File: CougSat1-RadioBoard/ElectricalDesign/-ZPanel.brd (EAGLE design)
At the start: 96 x 96 mm, 46 parts, among them J1 High Gain Antenna, J2 Deployables, J3 High Gain +, J4 ADCS, J5 Flap +X, J6 Flap -X, J7 Flap +Y, J8 Flap -Y, U1 AD7291, U3 AD8515

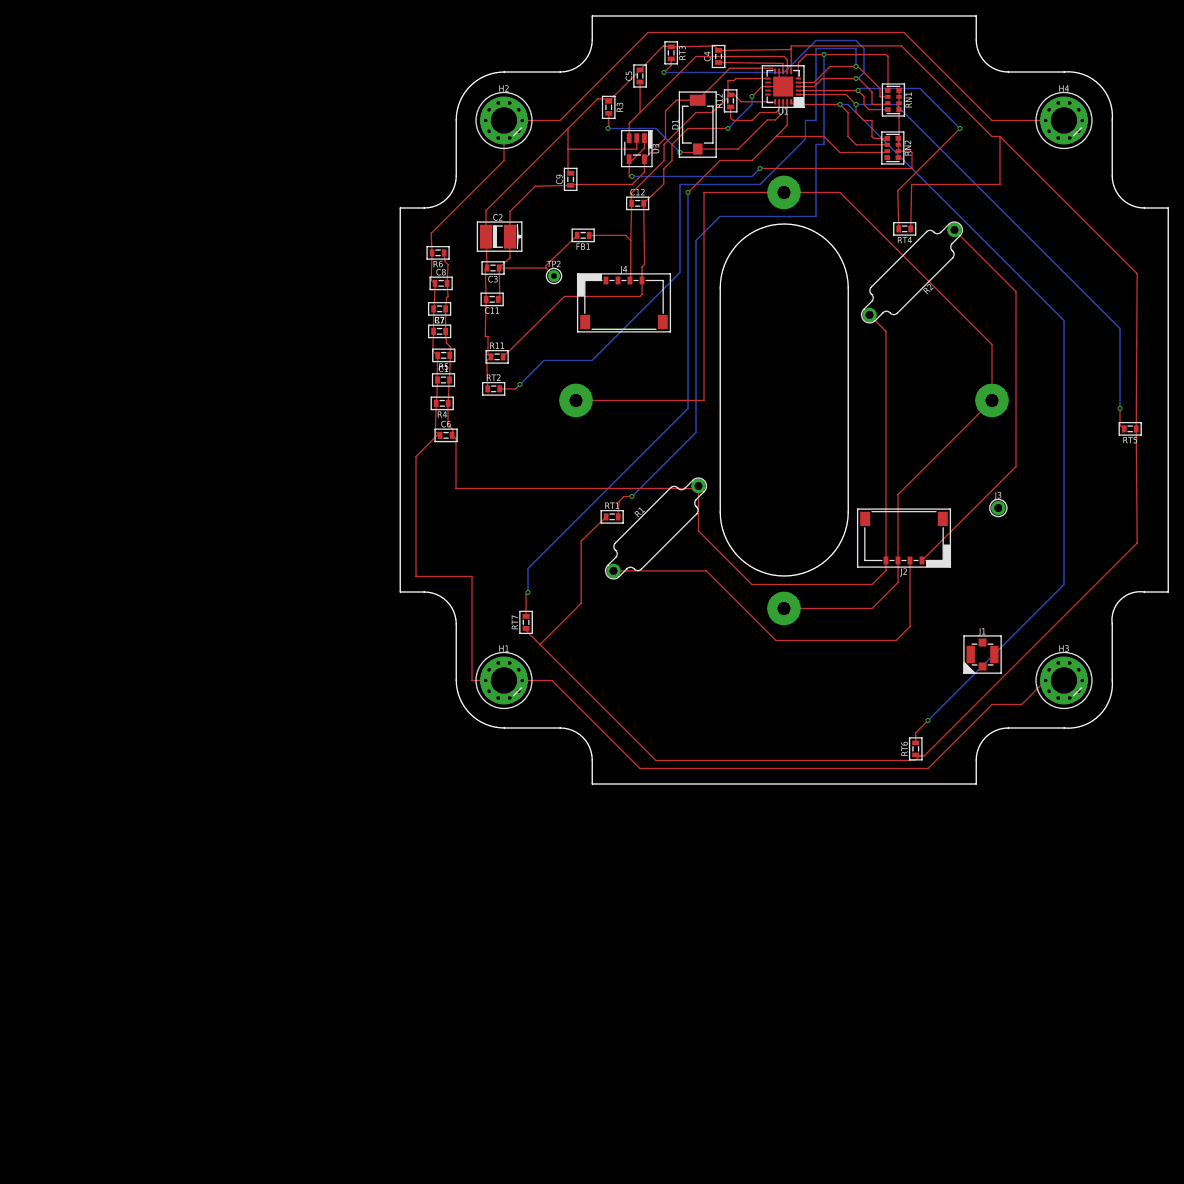
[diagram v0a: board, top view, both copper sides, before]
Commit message: Laid out RF
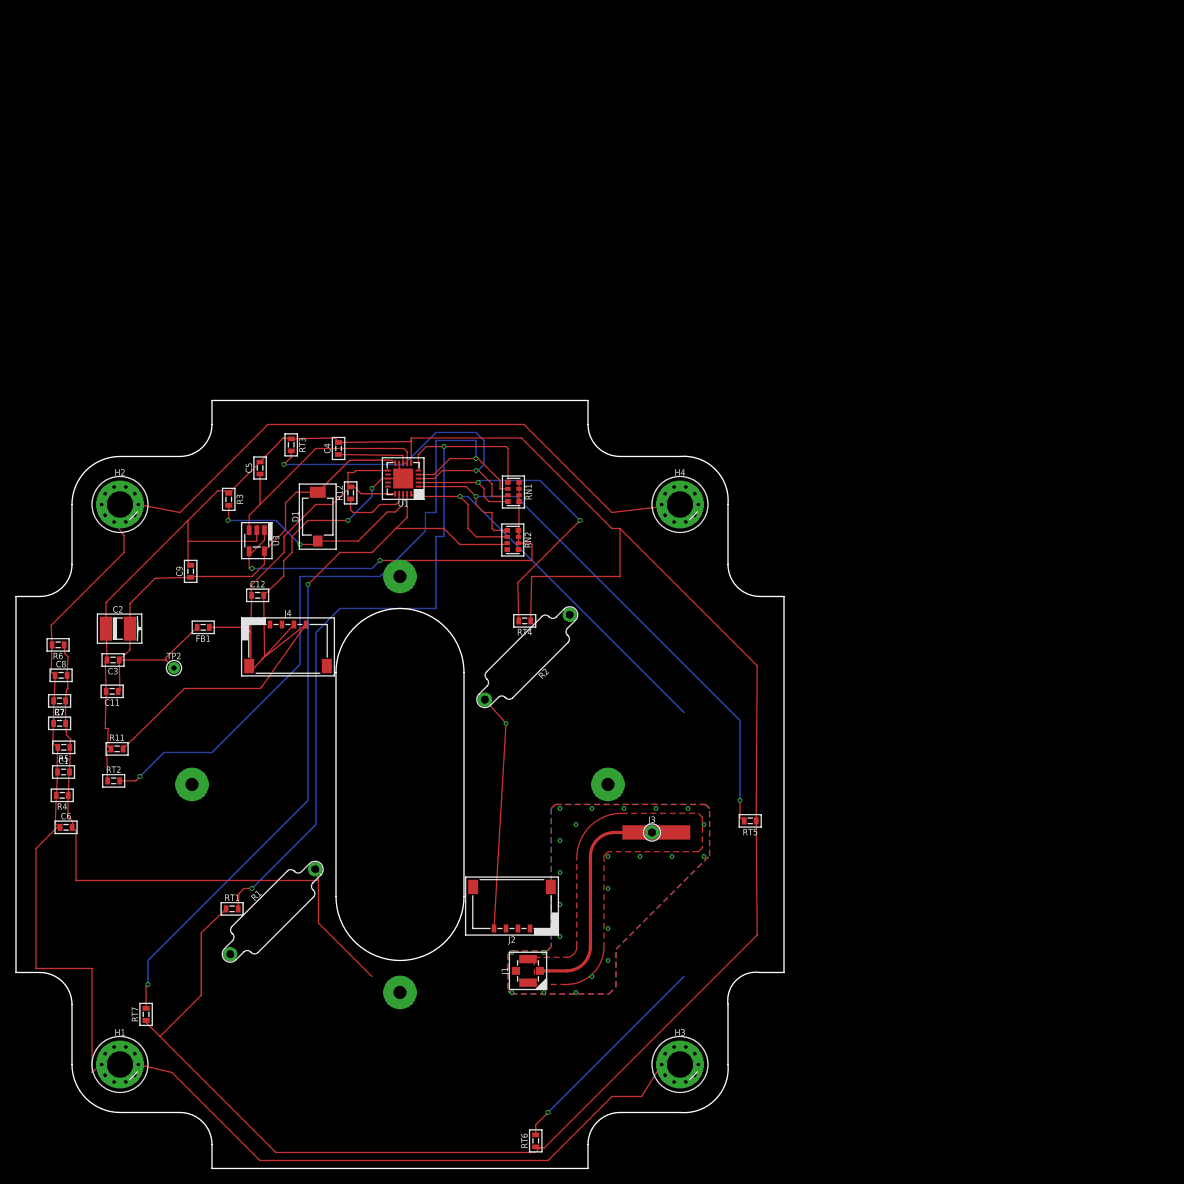
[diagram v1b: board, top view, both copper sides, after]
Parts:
- moved J6 104.7 mm to (-26.0, 0.00)
- moved J8 104.7 mm to (0.00, -26.0)
- moved J1 69.2 mm to (16.0, -23.3), turned to 90 degrees
- moved C1 68.2 mm to (-42.1, 1.56)
- moved C11 68.2 mm to (-36.0, 11.6)
- moved C12 68.2 mm to (-17.8, 23.6)
- moved C2 68.2 mm to (-35.2, 19.5)
- moved C3 68.2 mm to (-35.9, 15.6)
- moved C4 68.2 mm to (-7.68, 42.0)
- moved C5 68.2 mm to (-17.5, 39.6)
- moved C6 68.2 mm to (-41.7, -5.36)
- moved C7 68.2 mm to (-42.5, 7.64)
- moved C8 68.2 mm to (-42.4, 13.6)
- moved C9 68.2 mm to (-26.2, 26.6)
- moved D1 68.2 mm to (-10.3, 33.5)
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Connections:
- net HIGH_G_1 renamed COAX_CENTER
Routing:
- net SPRING_CONTACT: track 136.1 -> 0.00 mm
- net DEPLOY-H: track 99.0 -> 0.00 mm
- net THERM-5: track 115.6 -> 82.6 mm
- net COAX_CENTER: track 0.00 -> 27.8 mm
- net PGND: track 126.2 -> 106.7 mm, vias 0 -> 1
- net DGND: track 60.5 -> 73.6 mm
- net 3.3V: track 48.1 -> 56.0 mm
- net CHASSIS: track 234.3 -> 236.5 mm
- added copper zone on layer 1, net RFGND
- added copper zone on layer 16, net RFGND
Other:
- outline, holes or cut-outs redrawn

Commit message: Update -ZPanel.brd
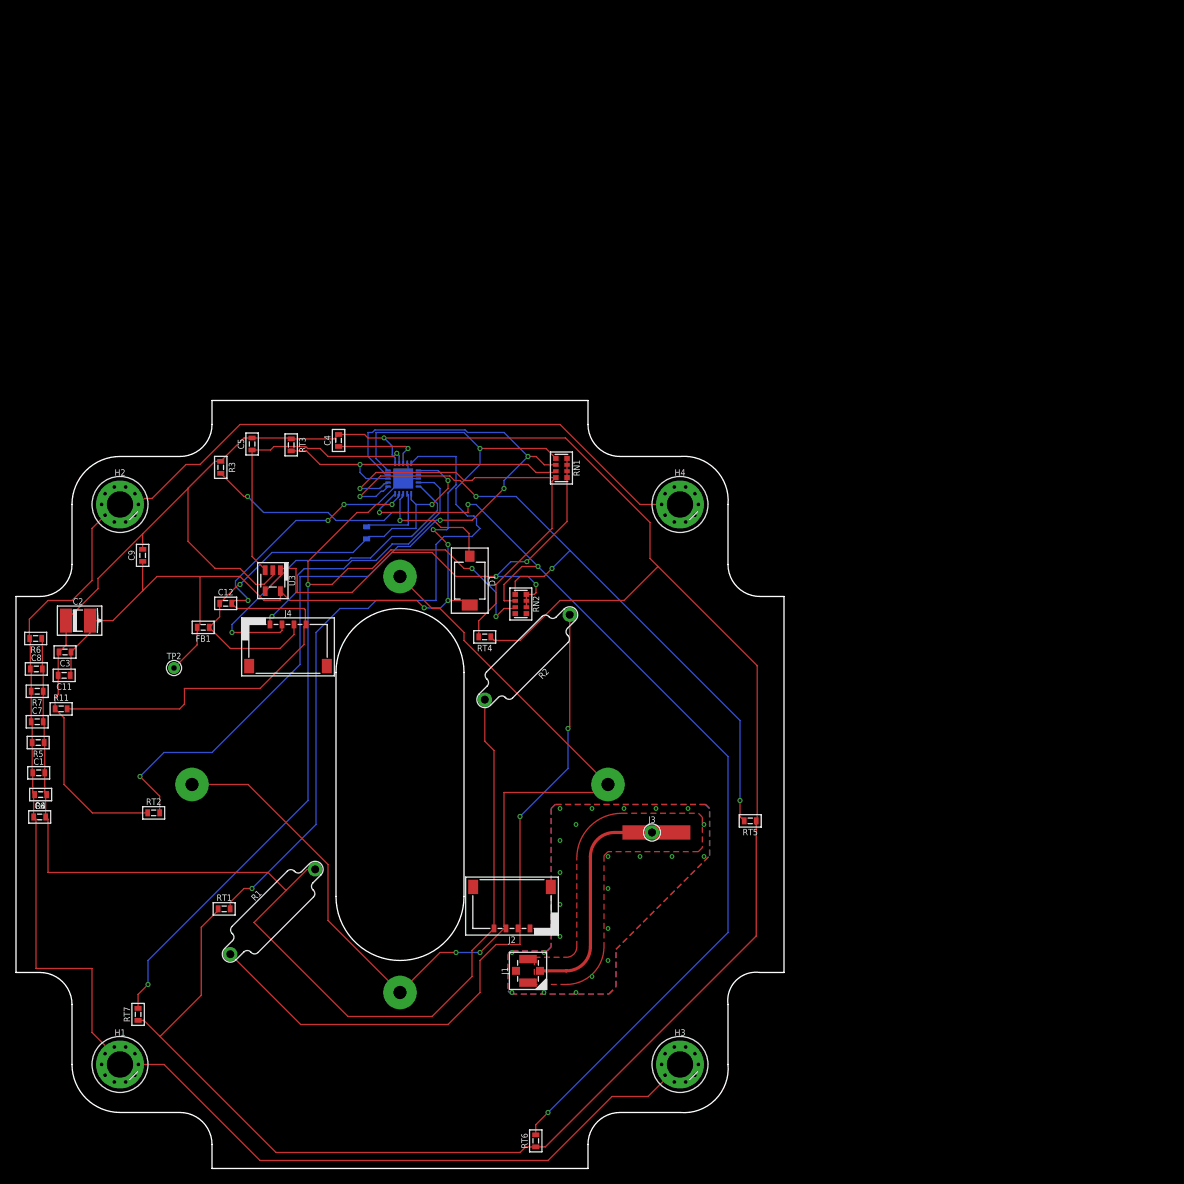
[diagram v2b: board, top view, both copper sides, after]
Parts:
- moved D1 20.6 mm to (8.72, 25.5), turned to 270 degrees
- moved R11 8.60 mm to (-42.4, 9.45)
- moved RN2 8.06 mm to (15.1, 22.6)
- moved RN1 6.71 mm to (20.2, 39.6)
- moved RT2 6.40 mm to (-30.8, -3.55)
- moved C11 6.32 mm to (-42.0, 13.6)
- moved C9 6.32 mm to (-32.2, 28.6)
- moved C3 6.08 mm to (-41.9, 16.6)
- moved R12 5.39 mm to (-4.17, 31.4), flipped to the bottom, turned to 270 degrees
- moved RT4 5.39 mm to (10.6, 18.4)
- moved U3 5.39 mm to (-15.9, 25.5)
- moved C2 5.10 mm to (-40.2, 20.5)
- moved C12 4.12 mm to (-21.8, 22.6)
- moved R3 4.12 mm to (-22.4, 39.6)
- moved C6 3.55 mm to (-45.0, -4.06)
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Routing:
- net SPRING_CONTACT: track 0.00 -> 125.3 mm, vias 0 -> 2
- net DEPLOY-H: track 0.00 -> 90.4 mm, vias 0 -> 2
- net THERM-5: track 82.6 -> 126.6 mm, vias 2 -> 4
- net I2C_SCL_ADCS: track 0.00 -> 43.8 mm, vias 0 -> 1
- net AVDD: track 68.3 -> 104.8 mm, vias 0 -> 4
- net I2C_SDA_ADCS: track 0.00 -> 34.7 mm, vias 0 -> 1
- net PGND: track 106.7 -> 141.3 mm, vias 1 -> 0
- net AGND: track 315.8 -> 344.7 mm, vias 0 -> 1
- net THERM-6: track 95.0 -> 113.2 mm, vias 2 -> 5
- net THERM-1: track 91.7 -> 109.6 mm, vias 2 -> 4
- net THERM-0: track 94.6 -> 111.7 mm
- net THERM-4: track 72.5 -> 88.1 mm, vias 2 -> 4
- net PHOTODIODE_ADC: track 28.5 -> 41.0 mm
- net AVREF: track 54.0 -> 65.7 mm, vias 2 -> 3
- net THERM-3: track 43.4 -> 53.6 mm, vias 2 -> 1
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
